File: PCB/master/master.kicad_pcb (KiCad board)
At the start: 2 copper layers, 88.9 x 88.9 mm, 25 parts, among them J1 Conn_01x04_Female, J2 Conn_01x04_Female, U1 Pico, U2 BOB-12009, U3 ULN2003, U4 BOB-12009

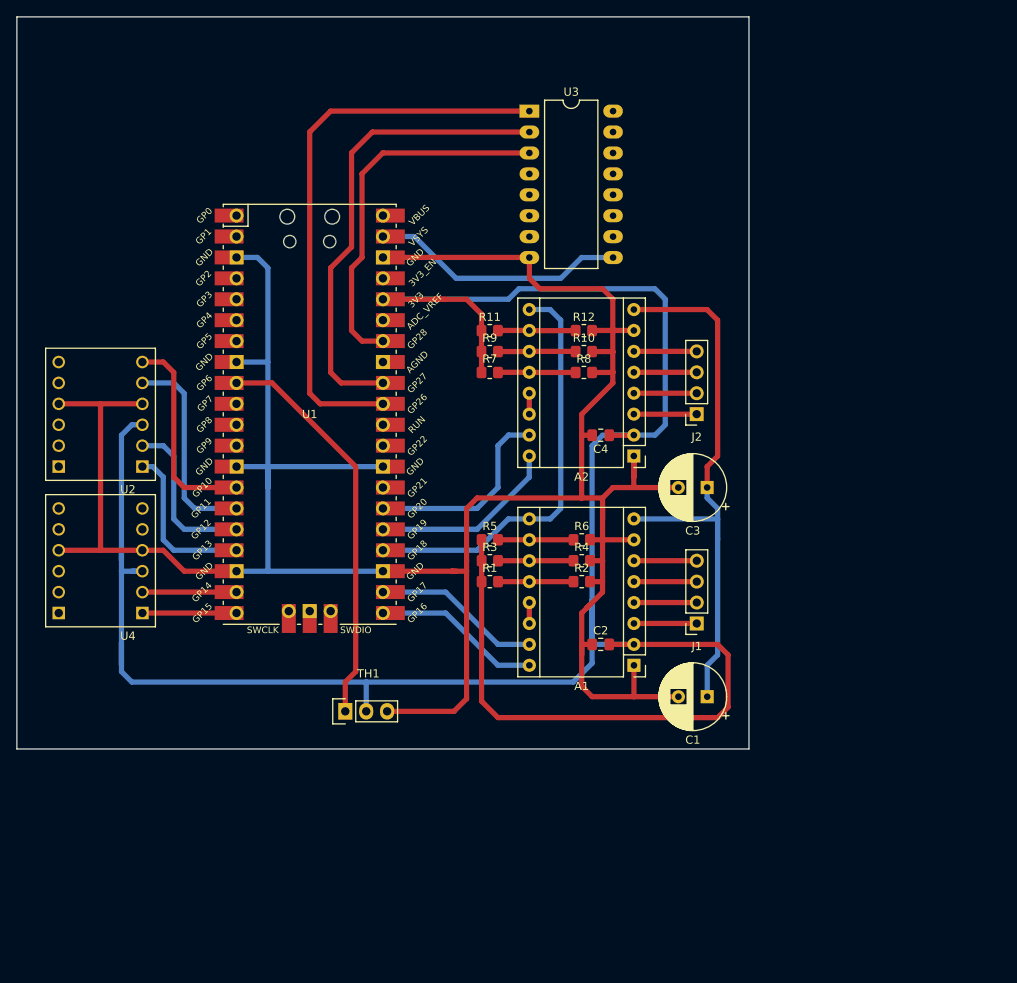
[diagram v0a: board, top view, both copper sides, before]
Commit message: if the tube stuck at printer reopen the lock
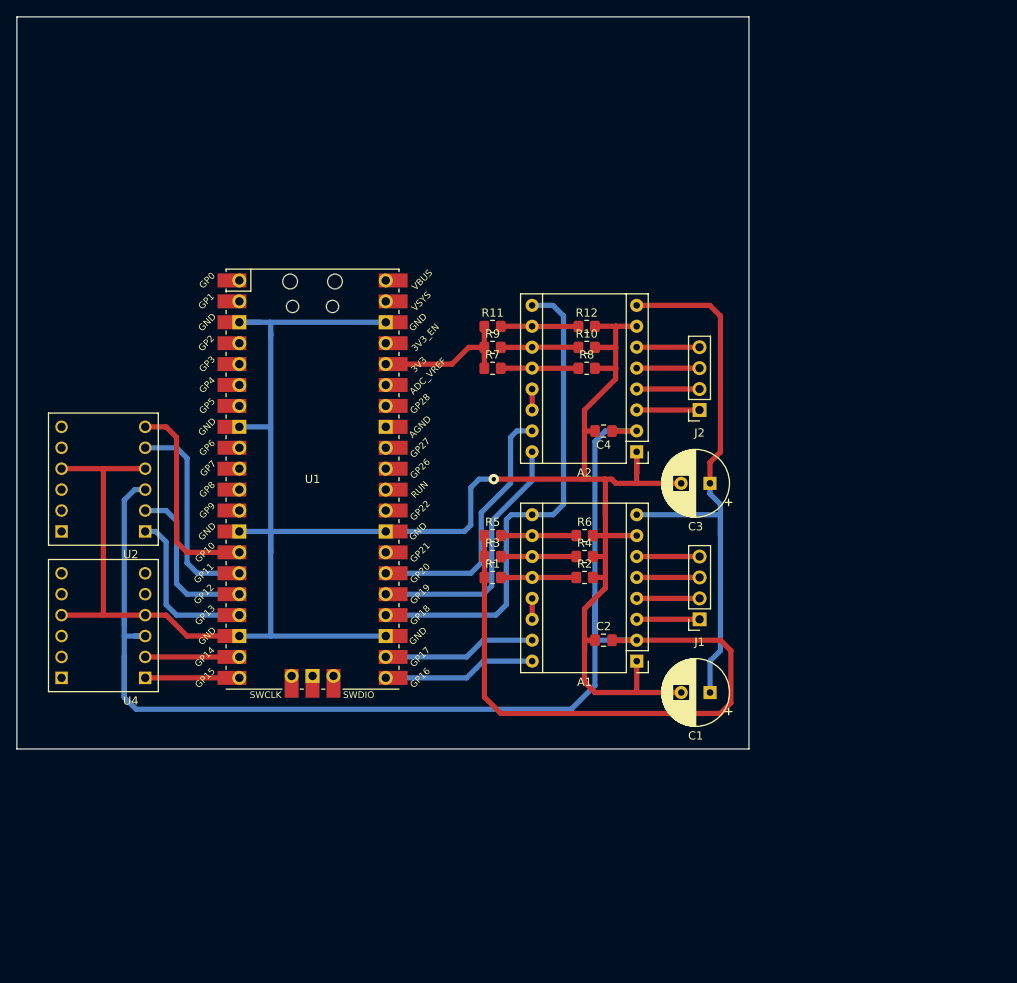
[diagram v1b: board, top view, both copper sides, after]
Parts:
- removed TH1: DHT11_Temperature_Humidity, Sensors:DHT11_Temperature_Humidity
- removed U3: ULN2003, Package_DIP:DIP-16_W10.16mm_LongPads
- moved U1 7.88 mm to (119.7, 81.5)
- moved U2 7.88 mm to (94.3, 81.5)
- moved U4 7.88 mm to (94.3, 99.3)
- moved R10 0.61 mm to (153.0, 65.5)
- moved R12 0.61 mm to (153.0, 63.0)
- moved C3 0.61 mm to (168.0, 82.0)
- moved J1 0.61 mm to (166.7, 98.6)
- moved R8 0.61 mm to (153.0, 68.1)
- moved C1 0.61 mm to (168.0, 107.4)
- moved C4 0.61 mm to (155.1, 75.7)
- moved R1 0.61 mm to (141.6, 93.5)
- moved R2 0.61 mm to (152.8, 93.5)
- moved R5 0.61 mm to (141.6, 88.4)
- moved R6 0.61 mm to (152.8, 88.4)
- moved R9 0.61 mm to (141.6, 65.5)
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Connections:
- U1 pad 31: Net-(U3-Pad1) -> unconnected-(U1-Pad31)
- U1 pad 32: Net-(U3-Pad2) -> unconnected-(U1-Pad32)
- U1 pad 34: Net-(U3-Pad3) -> unconnected-(U1-Pad34)
- U1 pad 9: /DHT_PIN -> unconnected-(U1-Pad9)
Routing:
- net Net-(U3-Pad1): track 68.9 -> 0.00 mm
- net +3V3: track 295.4 -> 234.8 mm
- net Net-(U3-Pad2): track 57.2 -> 0.00 mm
- net /DHT_PIN: track 48.9 -> 0.00 mm
- net GND: track 338.8 -> 291.8 mm, vias 0 -> 1
- net Net-(U3-Pad3): track 45.3 -> 0.00 mm
- net +5V: track 31.1 -> 0.00 mm
- net /Motor_EN: track 50.9 -> 60.4 mm
- net /M2_DIR: track 23.0 -> 31.6 mm
- net /M2_STEP: track 24.4 -> 31.8 mm
- net /M1_STEP: track 20.4 -> 18.6 mm
- net /M1_DIR: track 20.4 -> 18.6 mm

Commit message: update masters and printer
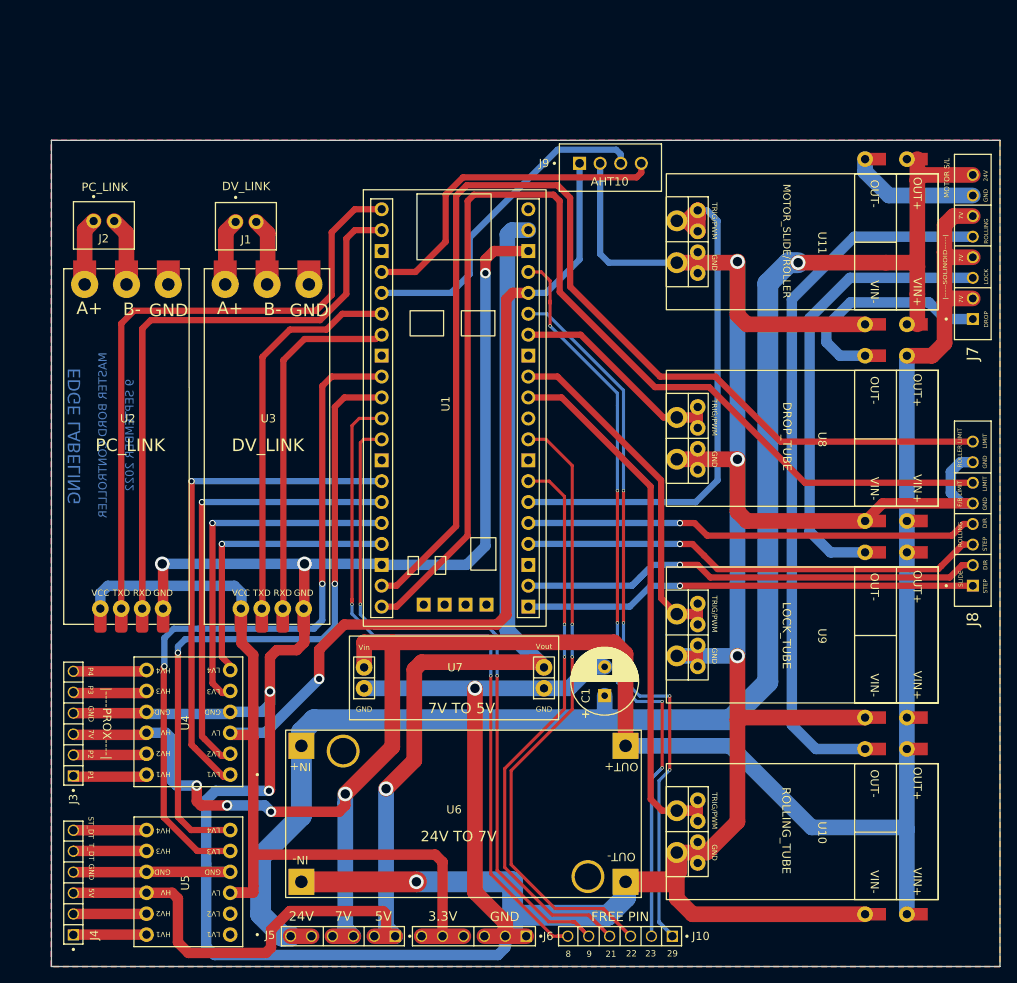
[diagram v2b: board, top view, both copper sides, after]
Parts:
- removed A1, A2: Pololu_Breakout_A4988, Module:Pololu_Breakout-16_15.2x20.3mm
- removed C2, C4: C_Small, Capacitor_SMD:C_0805_2012Metric_Pad1.18x1.45mm_HandSolder
- removed C3: C_Polarized, Capacitor_THT:CP_Radial_D8.0mm_P3.50mm
- removed R1, R10, R11, R12, R2, R3, R4, R5, R6, R7, R8, R9: R, Resistor_SMD:R_0805_2012Metric_Pad1.20x1.40mm_HandSolder
- added J10: 3-644456-6-6pin, 6pin:TE_3-644456-6, F.Cu at (163.4, 137.0)
- added J3: 3-644456-6-6pin, 6pin:TE_3-644456-6, F.Cu at (90.7, 117.6)
- added J4: 3-644456-6-6pin, 6pin:TE_3-644456-6, F.Cu at (90.7, 136.9)
- added J5: 3-644456-6-6pin, 6pin:TE_3-644456-6, F.Cu at (129.8, 137.0)
- added J6: 3-644456-6-6pin, 6pin:TE_3-644456-6, F.Cu at (145.7, 137.0)
- added J7: 177537-8, 8pin:TE_177537-8, F.Cu at (199.9, 53.3)
- added J8: 177537-8, 8pin:TE_177537-8, F.Cu at (199.9, 85.7)
- added J9: B4B-XH-A(LF)(SN), 4pin:JST_B4B-XH-A(LF)(SN), F.Cu at (152.1, 43.2)
- added U10: XY_Mos, XY_MOS:XY_MOS, F.Cu at (181.1, 124.5)
- added U11: XY_Mos, XY_MOS:XY_MOS, F.Cu at (181.1, 52.8)
- added U3: RS485_Module, RS485_MODULE:RS485_MODULE, F.Cu at (114.4, 74.7)
- added U5: 757, 4_CH_Shifter:4_CH_Shifter, F.Cu at (104.6, 130.6)
- added U6: 24V_TO_7V_43mm_x_20mm, Regurator_Module:24V_TO_7V_43mm_x_20mm, F.Cu at (137.3, 121.2)
- added U7: 7V_TO_5V_Module, Regurator_Module:7V_TO_5V_Module, F.Cu at (137.0, 104.9)
- added U8: XY_Mos, XY_MOS:XY_MOS, F.Cu at (181.1, 76.7)
- added U9: XY_Mos, XY_MOS:XY_MOS, F.Cu at (181.1, 100.6)
- C1: value C_Polarized -> C
- J1, J2: value Conn_01x04_Female -> B2B-XH-A(LF)(SN); footprint Connector_PinSocket_2.54mm:PinSocket_1x04_P2.54mm_Vertical -> 2pin:JST_B2B-XH-A(LF)(SN)
- U1: value Pico -> WeAct-RP2040-Pico; footprint MCU_RaspberryPi_and_Boards:RPi_Pico_SMD_TH -> RP2040_CHINA:RP2040_CHINA
- U2: value BOB-12009 -> RS485_Module; footprint MyJobs:CONV_BOB-12009 -> RS485_MODULE:RS485_MODULE
- U4: value BOB-12009 -> 757; footprint MyJobs:CONV_BOB-12009 -> 4_CH_Shifter:4_CH_Shifter
- moved J2 75.9 mm to (94.4, 50.2)
- moved J1 73.2 mm to (111.6, 50.3)
- moved U1 19.2 mm to (136.9, 72.9)
- moved U4 15.7 mm to (104.6, 111.1)
- moved C1 12.8 mm to (155.2, 107.8), turned to 90 degrees
- moved U2 7.47 mm to (97.3, 74.7), turned to 0 degrees
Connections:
- C1 pad 1: +24V -> 24V
- J2 pad 1: Net-(A2-Pad3) -> Net-(J2-Pad1)
- J2 pad 2: Net-(A2-Pad4) -> Net-(J2-Pad2)
- U1 pad 1: unconnected-(U1-Pad1) -> PC_LINK_PIN0
- U1 pad 10: unconnected-(U1-Pad10) -> ST_DT
- U1 pad 11: unconnected-(U1-Pad11) -> PIN_8
- U1 pad 12: unconnected-(U1-Pad12) -> PIN_9
- U1 pad 13: GND -> unconnected-(U1-Pad13)
- U1 pad 14: Net-(U1-Pad14) -> PROX1
- U1 pad 15: Net-(U1-Pad15) -> PROX2
- U1 pad 16: Net-(U1-Pad16) -> PROX3
- U1 pad 17: Net-(U1-Pad17) -> PROX4
- U1 pad 19: Net-(U1-Pad19) -> roller_limit
- U1 pad 2: unconnected-(U1-Pad2) -> PC_LINK_PIN1
- U1 pad 20: Net-(U1-Pad20) -> F/B_limit
- U1 pad 21: /M1_DIR -> Sliding_step
- U1 pad 22: /M1_STEP -> Sliding_DIR
- U1 pad 23: GND -> unconnected-(U1-Pad23)
- U1 pad 24: /Motor_EN -> Rolling_step
- U1 pad 25: /M2_DIR -> Rolling_DIR
- U1 pad 26: /M2_STEP -> Relay_Slide & Rolling
- U1 pad 27: unconnected-(U1-Pad27) -> PIN_21
- U1 pad 28: GND -> unconnected-(U1-Pad28)
- U1 pad 29: unconnected-(U1-Pad29) -> PIN_22
- U1 pad 3: GND -> unconnected-(U1-Pad3)
- U1 pad 31: unconnected-(U1-Pad31) -> Rolling_Solinoid
- U1 pad 32: unconnected-(U1-Pad32) -> Lock_Solinoid
- U1 pad 34: unconnected-(U1-Pad34) -> Drop_Solinoid
- U1 pad 35: unconnected-(U1-Pad35) -> PIN_29
- U1 pad 36: +3V3 -> 3.3V
- U1 pad 37: unconnected-(U1-Pad37) -> PIN_23
- U1 pad 39: +5V -> 5V
- U1 pad 4: unconnected-(U1-Pad4) -> SDA
- U1 pad 5: unconnected-(U1-Pad5) -> SCL
- U1 pad 6: unconnected-(U1-Pad6) -> DV_LINK_PIN4
- U1 pad 7: unconnected-(U1-Pad7) -> DV_LINK_PIN5
- U1 pad 8: GND -> unconnected-(U1-Pad8)
- U1 pad 9: unconnected-(U1-Pad9) -> TUBE_DT
- U4 pad HV: unconnected-(U4-PadHV) -> 7V
- U4 pad HV1: unconnected-(U4-PadHV1) -> Net-(J3-Pad1)
- U4 pad HV2: unconnected-(U4-PadHV2) -> Net-(J3-Pad2)
- U4 pad HV3: unconnected-(U4-PadHV3) -> Net-(J3-Pad5)
- U4 pad HV4: unconnected-(U4-PadHV4) -> Net-(J3-Pad6)
- U4 pad LV: +3V3 -> 3.3V
- U4 pad LV1: Net-(U1-Pad20) -> PROX1
- U4 pad LV2: Net-(U1-Pad19) -> PROX2
- U4 pad LV3: unconnected-(U4-PadLV3) -> PROX3
- U4 pad LV4: unconnected-(U4-PadLV4) -> PROX4
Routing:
- net GND: track 291.8 -> 602.1 mm, vias 1 -> 10
- net 7V: track 0.00 -> 267.7 mm, vias 0 -> 4
- net +3V3: track 234.8 -> 0.00 mm
- net 3.3V: track 0.00 -> 204.4 mm, vias 0 -> 1
- net 24V: track 0.00 -> 188.7 mm, vias 0 -> 1
- net 5V: track 0.00 -> 160.7 mm, vias 0 -> 1
- net F/B_limit: track 0.00 -> 137.3 mm
- net roller_limit: track 0.00 -> 134.7 mm
- net PIN_23: track 0.00 -> 112.0 mm, vias 0 -> 5
- net PC_LINK_PIN1: track 0.00 -> 106.8 mm
- net PIN_29: track 0.00 -> 89.8 mm, vias 0 -> 4
- net PIN_9: track 0.00 -> 88.3 mm, vias 0 -> 2
- net TUBE_DT: track 0.00 -> 87.9 mm, vias 0 -> 2
- net PIN_8: track 0.00 -> 87.5 mm, vias 0 -> 2
- net Rolling_tube: track 0.00 -> 86.9 mm
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- added copper zone on B.Cu, net GND
- added copper zone on F.Cu, net GND
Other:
- board size 88.9 x 88.9 mm -> 115.2 x 100.3 mm
- board text added: "21"
- board text added: "22"
- board text added: "23"
- board text added: "24V"
- board text added: "24V TO 7V"
- board text added: "29"
- board text added: "3.3V"
- board text added: "5V"
- board text added: "7V"
- board text added: "7V TO 5V"
- board text added: "8"
- board text added: "9"
- board text added: "AHT10"
- board text added: "DIR"
- board text added: "DROP"
- board text added: "DROP_TUBE"
- board text added: "DV_LINK"
- board text added: "EDGE LABELING"
- board text added: "F/B LIMIT"
- board text added: "FREE PIN"
- board text added: "GND"
- board text added: "LIMIT"
- board text added: "LOCK"
- board text added: "LOCK_TUBE"
- board text added: "MASTER BORD CONTROLLER 9 SEPTEMBER 2022"
- board text added: "MOTOR S/L"
- board text added: "MOTOR_SLIDE/ROLLER"
- board text added: "P1"
- board text added: "P2"
- board text added: "P3"
- board text added: "P4"
- board text added: "PC_LINK"
- board text added: "ROLLER LIMIT"
- board text added: "ROLLING"
- board text added: "ROLLING_TUBE"
- board text added: "SLIDE"
- board text added: "STEP"
- board text added: "ST_DT"
- board text added: "T_DT"
- board text added: "|-----SOLINOID-----|"
- board text added: "|----PROX----|"
